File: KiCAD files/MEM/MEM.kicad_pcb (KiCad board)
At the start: 2 copper layers, 99.7 x 69.8 mm, 28 parts, among them J1 card addr, J2 Power Bus, J3 Signal Bus, J4 RAM bank, J5 ROM block, U1 74LS139, U2 74LS04, U3 74LS74, U4 74LS85, U5 SN74LS07N, U6 628128, U7 W27C512

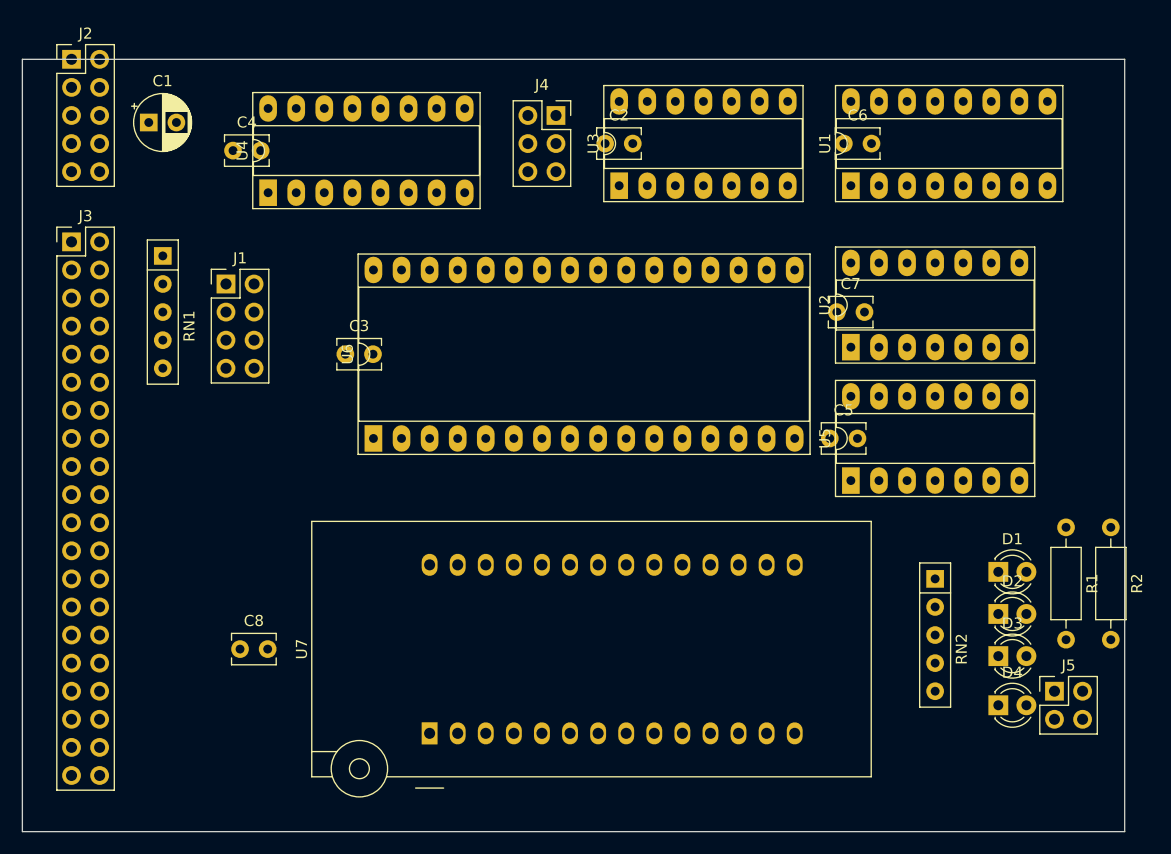
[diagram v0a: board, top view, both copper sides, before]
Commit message: home
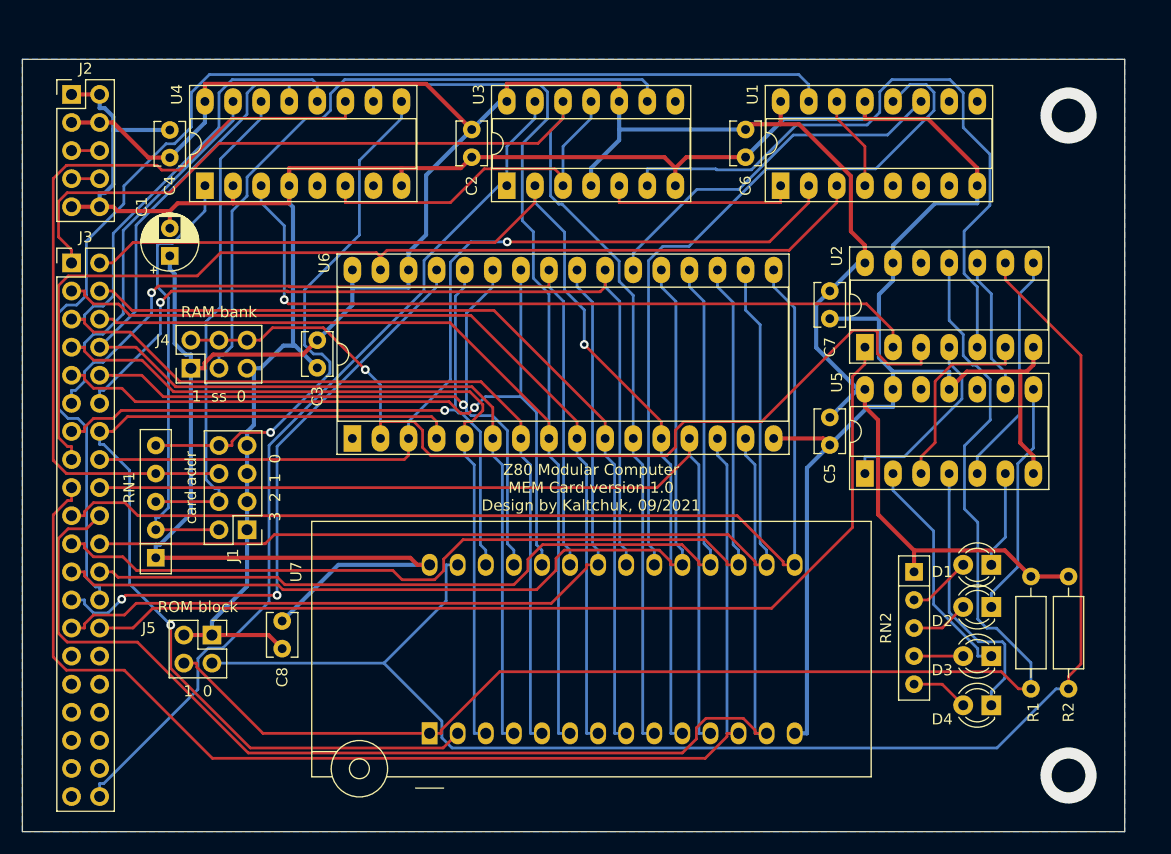
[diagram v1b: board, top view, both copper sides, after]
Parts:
- J4: footprint Connector_PinSocket_2.54mm:PinSocket_2x03_P2.54mm_Vertical -> Connector_PinHeader_2.54mm:PinHeader_2x03_P2.54mm_Vertical
- moved J5 76.4 mm to (115.6, 108.0), turned to 270 degrees
- moved J4 40.2 mm to (113.7, 83.8), turned to 90 degrees
- moved RN1 27.3 mm to (110.5, 101.0), turned to 90 degrees
- moved J1 22.3 mm to (118.7, 98.4), turned to 180 degrees
- moved C1 12.2 mm to (111.8, 73.7), turned to 90 degrees
- moved C2 12.1 mm to (139.1, 62.2), turned to 270 degrees
- moved U3 10.2 mm to (142.2, 67.3)
- moved C6 8.98 mm to (163.8, 62.2), turned to 270 degrees
- moved U1 6.35 mm to (167.0, 67.3)
- moved R2 5.86 mm to (193.0, 102.7)
- moved U4 5.75 mm to (114.9, 67.3)
- moved C4 5.75 mm to (111.8, 64.8), turned to 90 degrees
- moved R1 5.46 mm to (189.6, 102.7)
- moved C8 4.58 mm to (121.9, 106.7), turned to 270 degrees
- moved J2 3.17 mm to (102.9, 59.1)
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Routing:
- net GND: track 0.00 -> 276.2 mm
- net +5V: track 0.00 -> 269.0 mm
- net Net-(J5-Pad2): track 0.00 -> 137.8 mm
- net Net-(J5-Pad4): track 0.00 -> 126.8 mm
- net /a04: track 0.00 -> 124.9 mm
- net /a01: track 0.00 -> 118.6 mm
- net /mreq: track 0.00 -> 112.6 mm
- net /a05: track 0.00 -> 112.6 mm
- net /d02: track 0.00 -> 112.4 mm
- net /d01: track 0.00 -> 111.2 mm
- net /a06: track 0.00 -> 102.8 mm
- net /a07: track 0.00 -> 101.2 mm
- net /a00: track 0.00 -> 98.8 mm, vias 0 -> 1
- net /d03: track 0.00 -> 96.1 mm
- net /a15: track 0.00 -> 93.0 mm
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- added copper zone on B.Cu, net GND
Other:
- net class Power added: clearance 0.2, trace_width 0.375, via_dia 0.8, via_drill 0.4
- board text added: "1 0"
- board text added: "1 ss 0"
- board text added: "3 2 1 0"
- board text added: "RAM bank"
- board text added: "ROM block"
- board text added: "Z80 Modular Computer MEM Card version 1.0 Design by Kaltchuk, 09/2021"
- board text added: "card addr"
